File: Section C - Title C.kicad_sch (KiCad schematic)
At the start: 98 parts, among them J16 OSTOQ025450, J17 OSTOQ025450, J18 OSTOQ025450, J19 OSTOQ025450, J20 OSTOQ025450, J21 OSTOQ025450, J22 OSTOQ025450, J23 OSTOQ025450, J24 OSTOQ025450, J5 OSTOQ025450, K1 OJE-SH-105LMH,000, K10 OJE-SH-105LMH,000, K11 VOR1003M4T, K12 VOR1003M4T, K13 VOR1003M4T, K14 VOR1003M4T, K15 VOR1003M4T, K16 VOR1003M4T, K17 VOR1003M4T, K18 VOR1003M4T, K19 VOR1003M4T, K2 OJE-SH-105LMH,000, K20 VOR1003M4T, K3 OJE-SH-105LMH,000, K4 OJE-SH-105LMH,000, K5 OJE-SH-105LMH,000, K6 OJE-SH-105LMH,000, K7 OJE-SH-105LMH,000, K8 OJE-SH-105LMH,000, K9 OJE-SH-105LMH,000, Q10 IRLML2060, Q11 IRLML2060, Q12 IRLML2060, Q14 IRLML2060, Q15 IRLML2060, Q16 IRLML2060, Q17 IRLML2060, Q23 IRLML2060, Q24 IRLML2060, Q27 DMP6185SEQ-13, Q28 IRLML2060, Q29 IRLML2060, Q30 DMP6185SEQ-13, Q31 IRLML2060, Q32 DMP6185SEQ-13, Q33 IRLML2060, Q34 DMP6185SEQ-13, Q9 IRLML2060, T39 TestPoint, T40 TestPoint, T41 TestPoint, T42 TestPoint

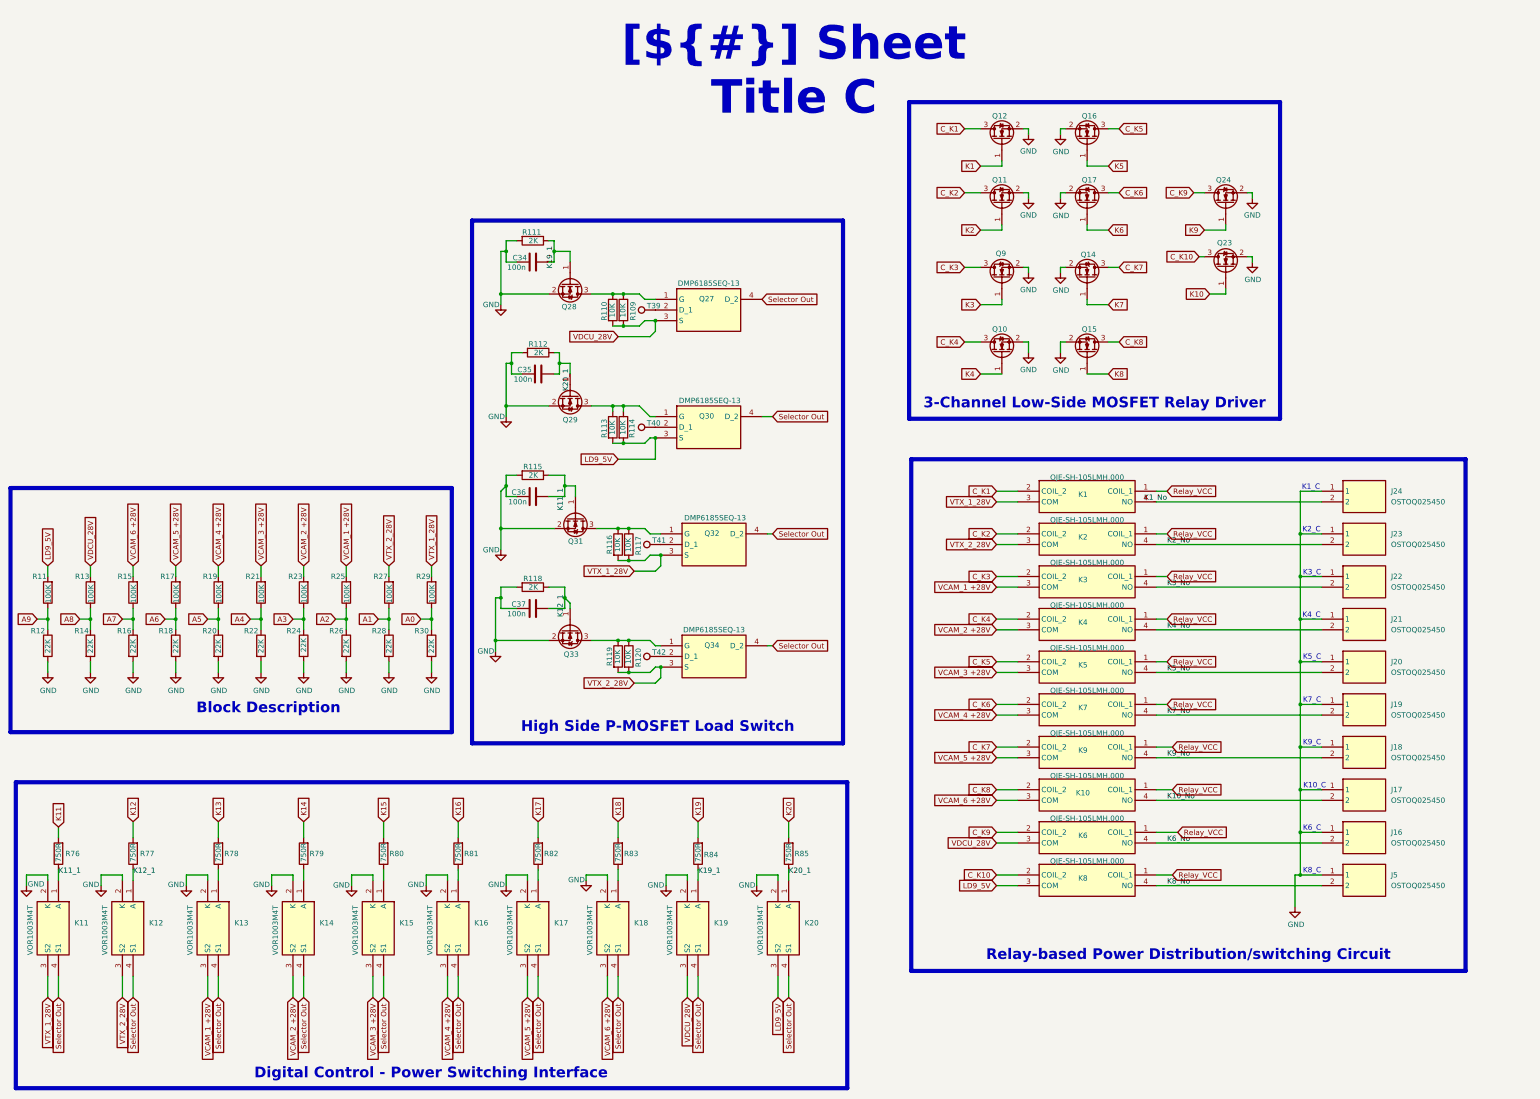
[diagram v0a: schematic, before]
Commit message: PCB Preliminary version
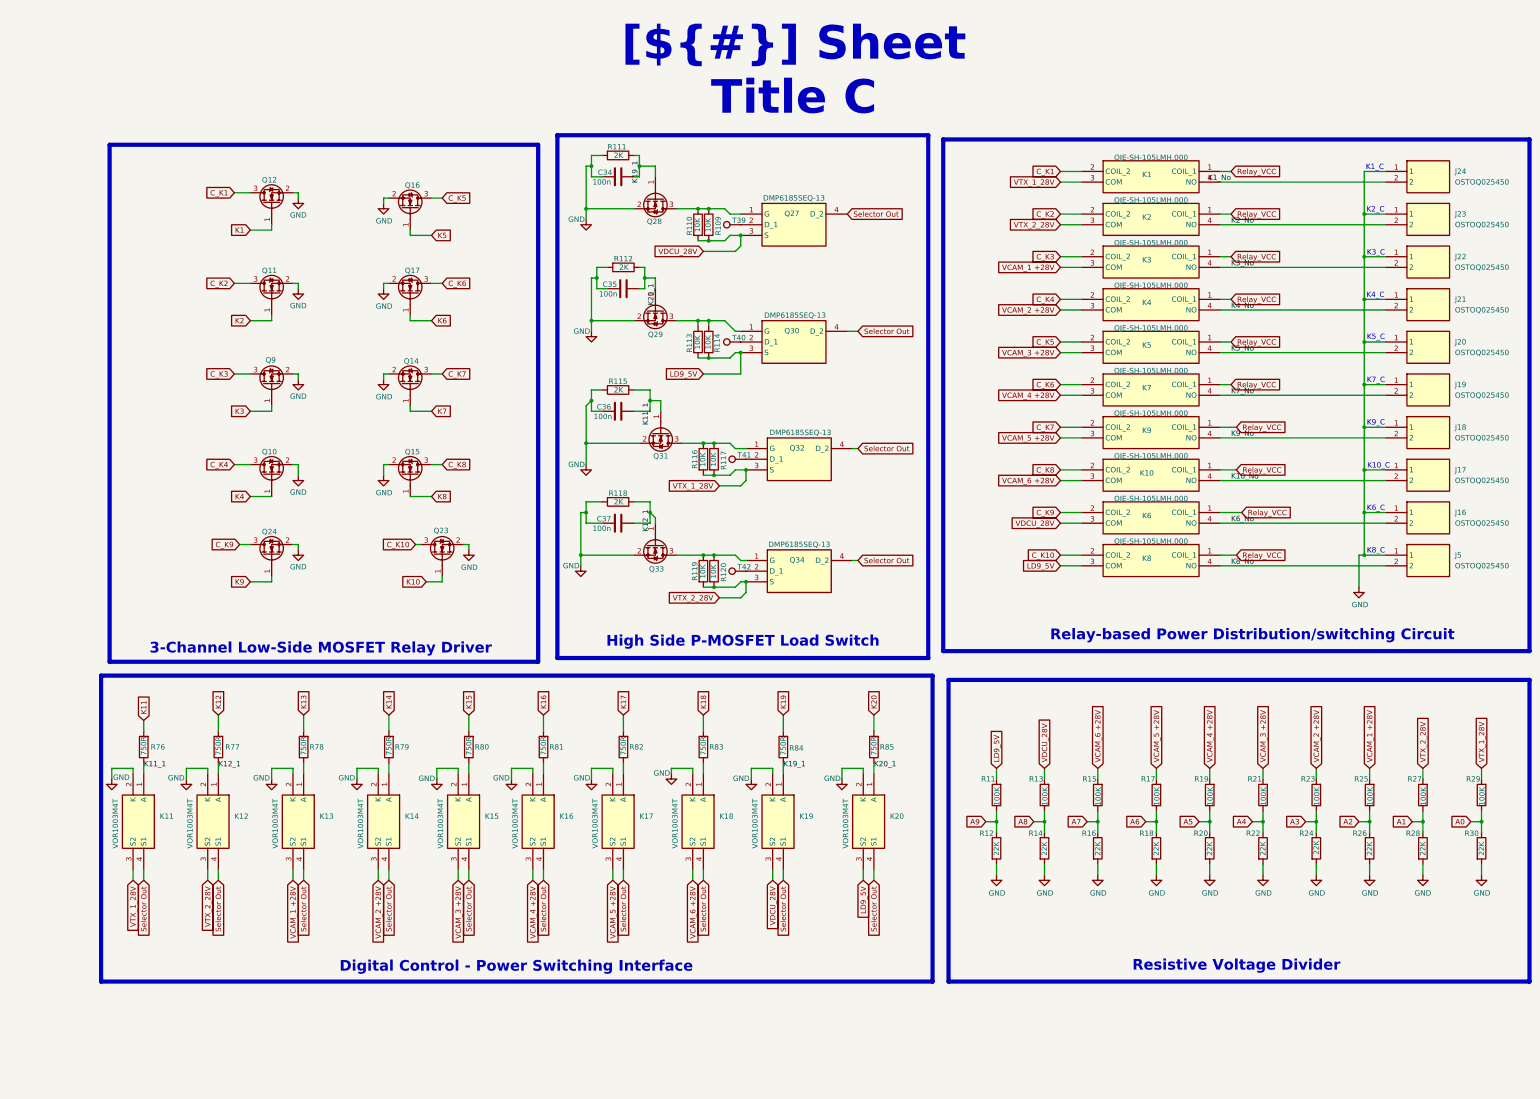
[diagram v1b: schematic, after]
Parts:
- T39, T40, T41, T42: footprint SamacSys_Parts:TestPoint_Pad_0.6x0.6mm -> TestPoint:TestPoint_Pad_1.0x1.0mm
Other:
- moved on the sheet: C34, C35, C36, C37, J16, J17, J18, J19, J20, J21, J22, J23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
